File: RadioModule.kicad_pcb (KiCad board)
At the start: 4 copper layers, 16 x 18 mm, 43 parts, among them J1 Conn_01x01_Pin, J10 Conn_01x01_Pin, J11 Conn_01x01_Pin, J12 Conn_01x01_Pin, J13 Conn_01x01_Pin, J14 Conn_01x01_Pin, J15 Conn_01x01_Pin, J16 Conn_01x01_Pin, J2 Conn_01x01_Pin, J3 Conn_01x01_Pin, J4 Conn_01x01_Pin, J5 Conn_01x01_Pin, J6 Conn_01x01_Pin, J7 Conn_01x01_Pin, J8 Conn_01x01_Pin, J9 Conn_01x01_Pin, U1 SX1280IMLTRT, Y1 ABM13W-52.0MHz

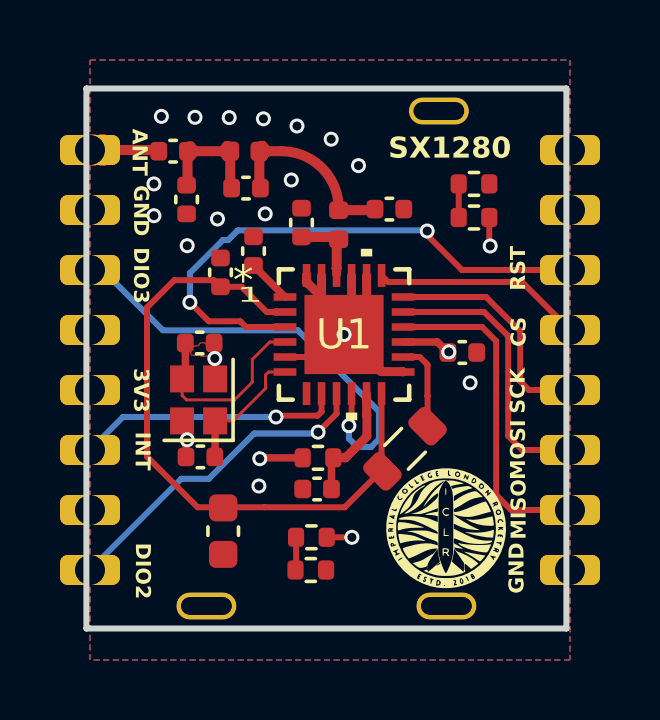
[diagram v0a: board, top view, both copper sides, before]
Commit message: Final Commit V1.0
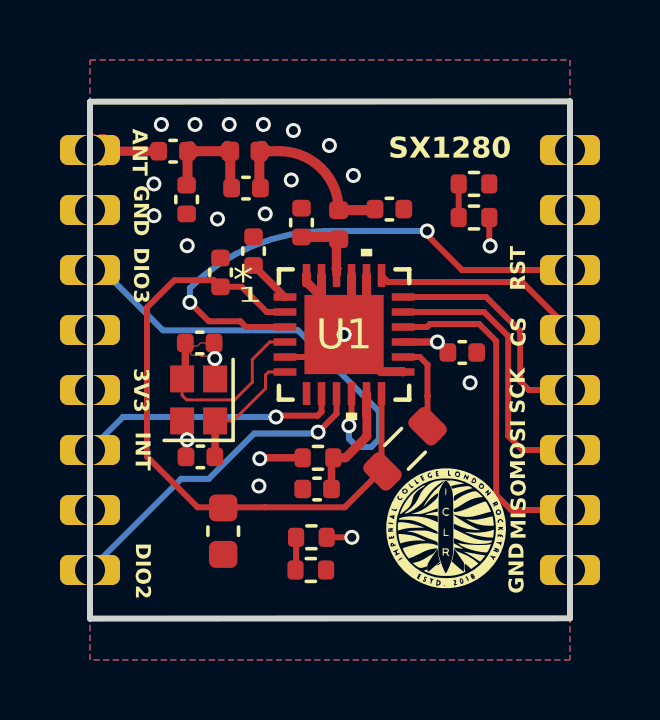
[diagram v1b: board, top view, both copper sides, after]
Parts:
- removed the ? at (93.9, 86.2)
- removed the ? at (101.9, 86.2)
- added ?: , , F.Cu at (101.9, 86.0)
- added ?: , , F.Cu at (93.9, 86.0)
- moved ? 0.45 mm to (101.6, 70.2)
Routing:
- net NRST: track 18.4 -> 17.8 mm
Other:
- board size 16 x 18 mm -> 16 x 17.2 mm

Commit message: Moved a via
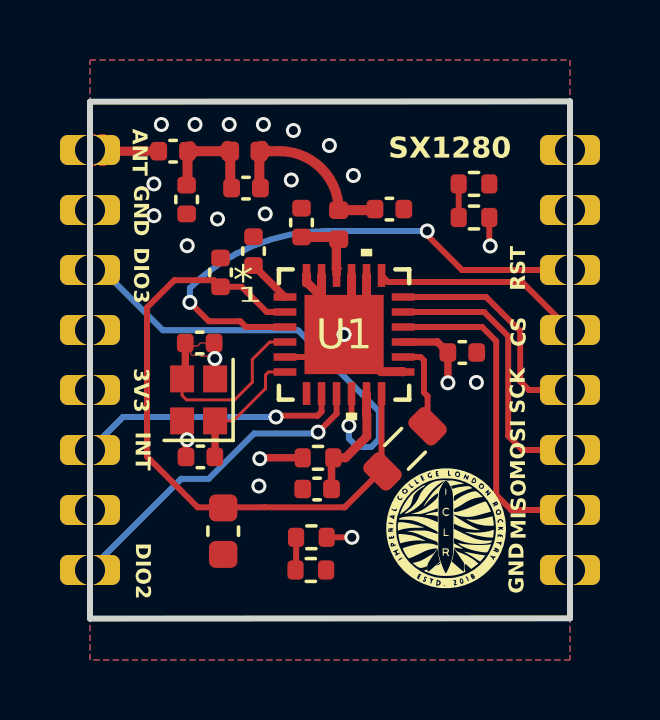
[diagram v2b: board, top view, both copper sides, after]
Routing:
- net 3V3: track 4.88 -> 5.89 mm
